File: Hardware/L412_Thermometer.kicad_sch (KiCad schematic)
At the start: 22 parts, among them J1 USB_B_Mini, J2 Conn_01x03, J3 Conn_Si7021, J4 Conn_LCD, J5 Debug, J6 Serial, U1 AP7343D-33W5, U2 STM32L412KBTx, Y1 ABS07 [9pF, 32.768kHz]

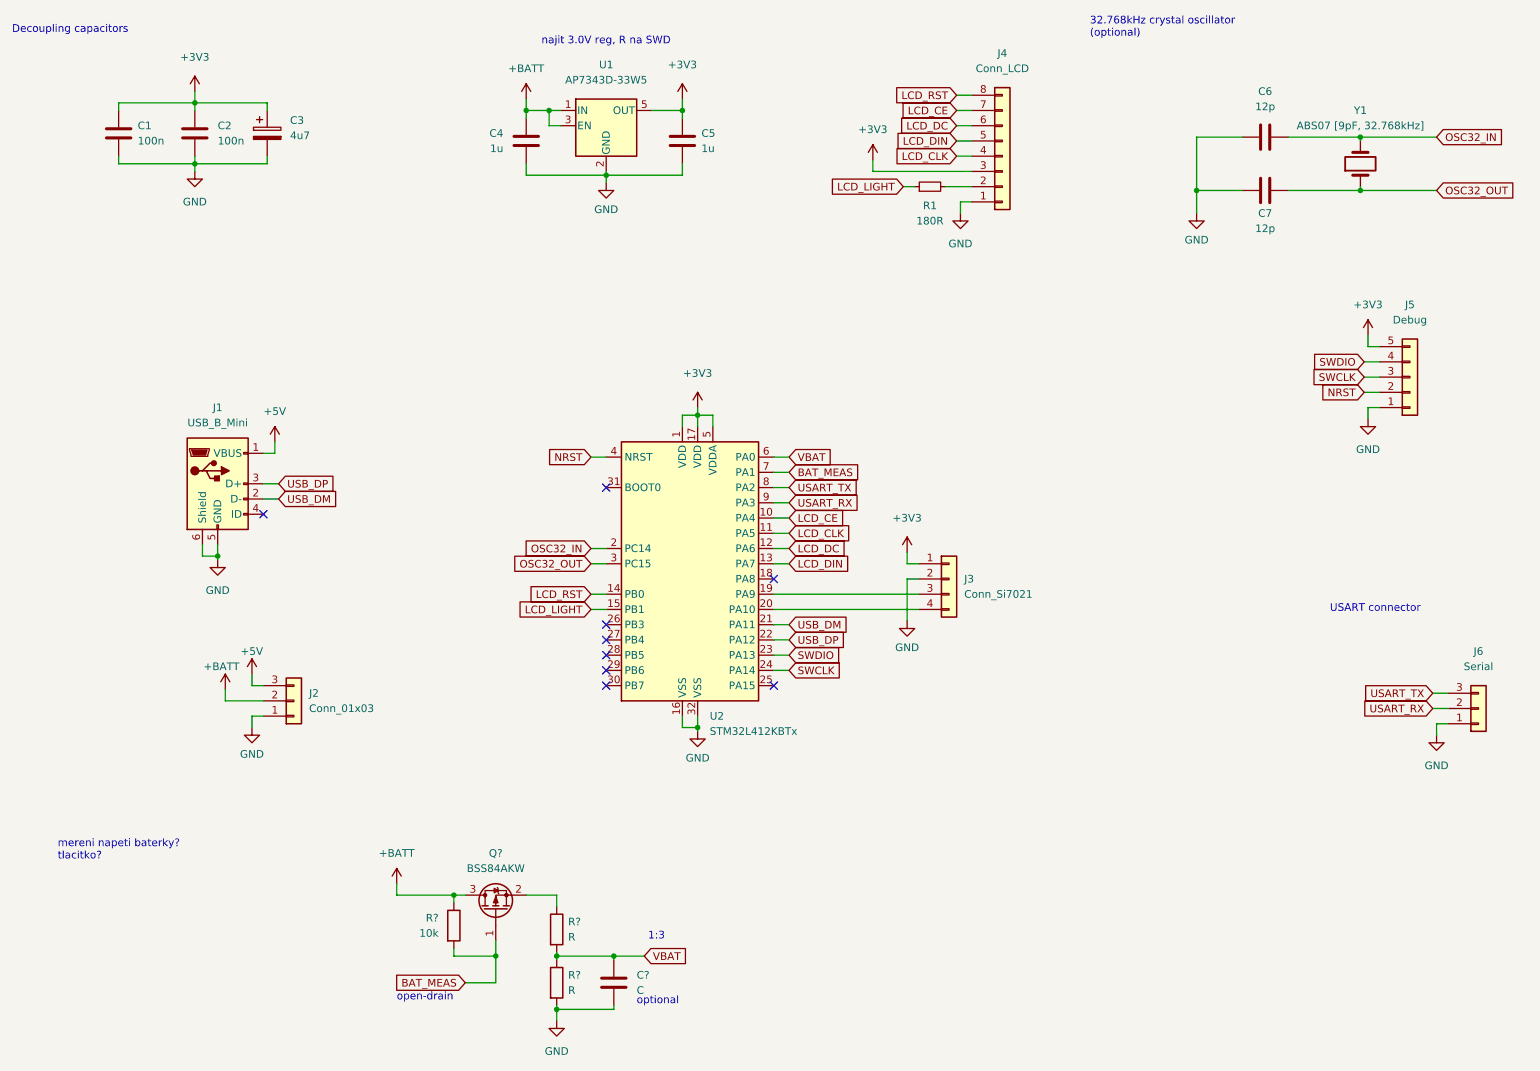
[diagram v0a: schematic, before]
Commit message: PCB updated
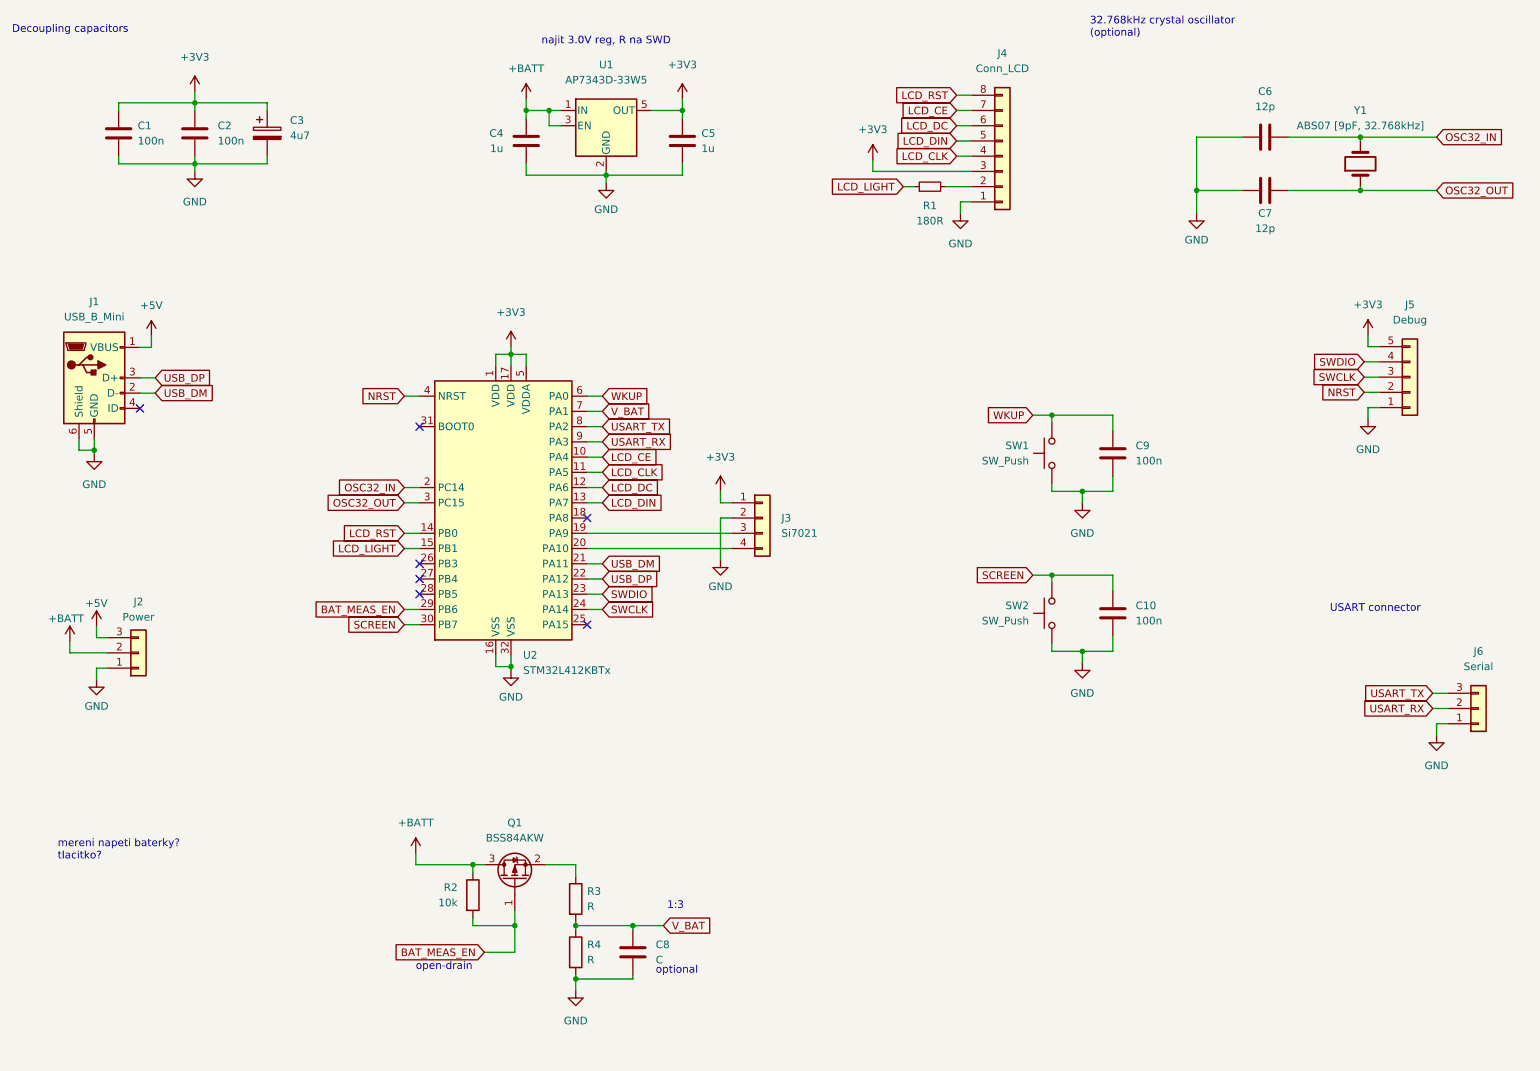
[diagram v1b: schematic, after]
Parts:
- added C10, C9: 100n, Capacitor_SMD:C_0603_1608Metric, symbol Device:C
- added SW1, SW2: SW_Push, Button_Switch_THT:SW_PUSH_6mm, symbol Switch:SW_Push
- C8: renamed from C?; footprint (none) -> Capacitor_SMD:C_0603_1608Metric
- J2: value Conn_01x03 -> Power
- J3: value Conn_Si7021 -> Si7021
- Q1: renamed from Q?; footprint (none) -> Package_TO_SOT_SMD:SOT-323_SC-70
- R2, R3, R4: renamed from R?; footprint (none) -> Resistor_SMD:R_0603_1608Metric
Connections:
- net GND: now also C10.2, C9.2, SW1.1, SW2.1
- net BAT_MEAS_EN: now reaches U2.29 (PB6)
- net BAT_MEAS_EN: now also Q1.1 (G), R2.2
- net SCREEN: now reaches U2.30 (PB7)
- net SCREEN: now also C10.1, SW2.2
- removed net BAT_MEAS: Q1.1 (G), R2.2, U2.7 (PA1)
- net VBAT renamed V_BAT
- net V_BAT: now also U2.7 (PA1); no longer U2.6 (PA0)
- new net WKUP: C9.1, SW1.2, U2.6 (PA0)
- no-connect marks 9 -> 7
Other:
- moved on the sheet: C8, J1, J2, J3, Q1, R2, R3, R4, U2
